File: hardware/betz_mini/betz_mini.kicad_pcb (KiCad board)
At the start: 2 copper layers, 17 parts, among them U1 stm32g474ceu6, U2 AS5047U, U3 IIS328DQ, U4 MP6540

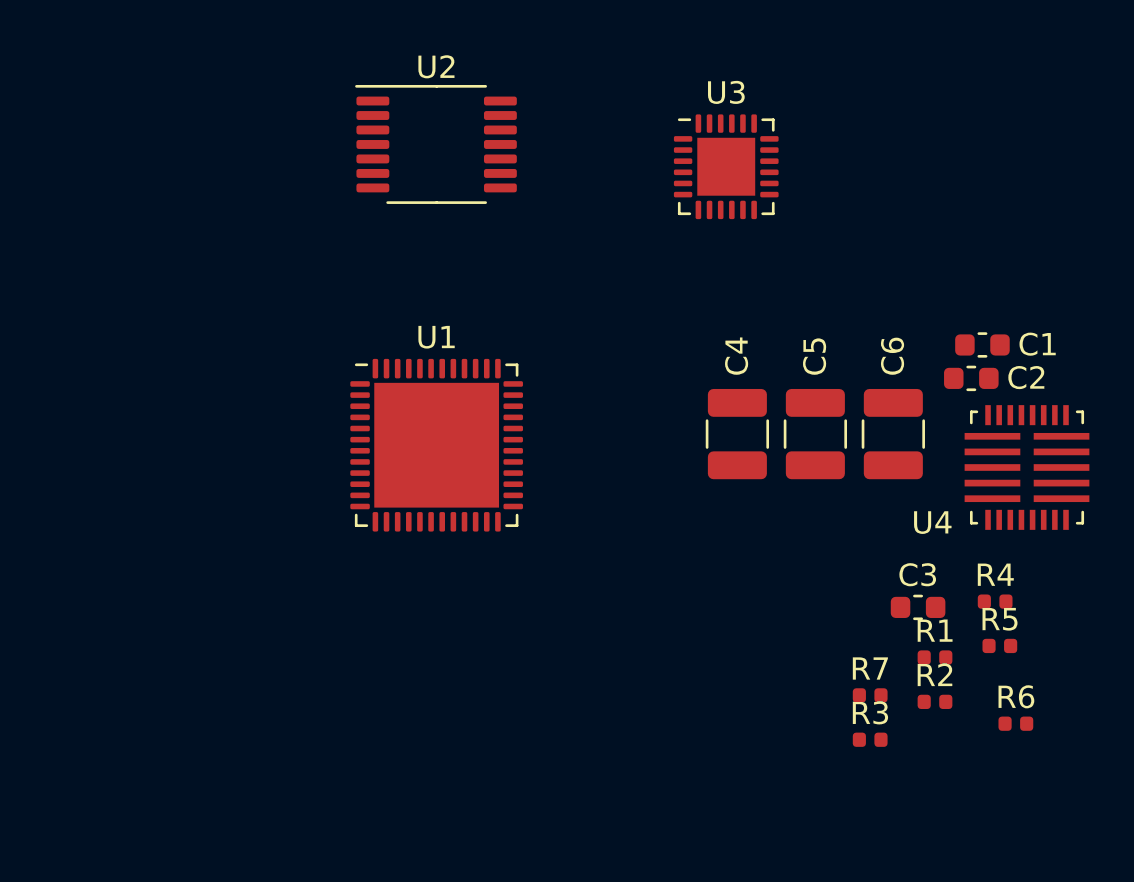
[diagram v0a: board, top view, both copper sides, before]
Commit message: WIP
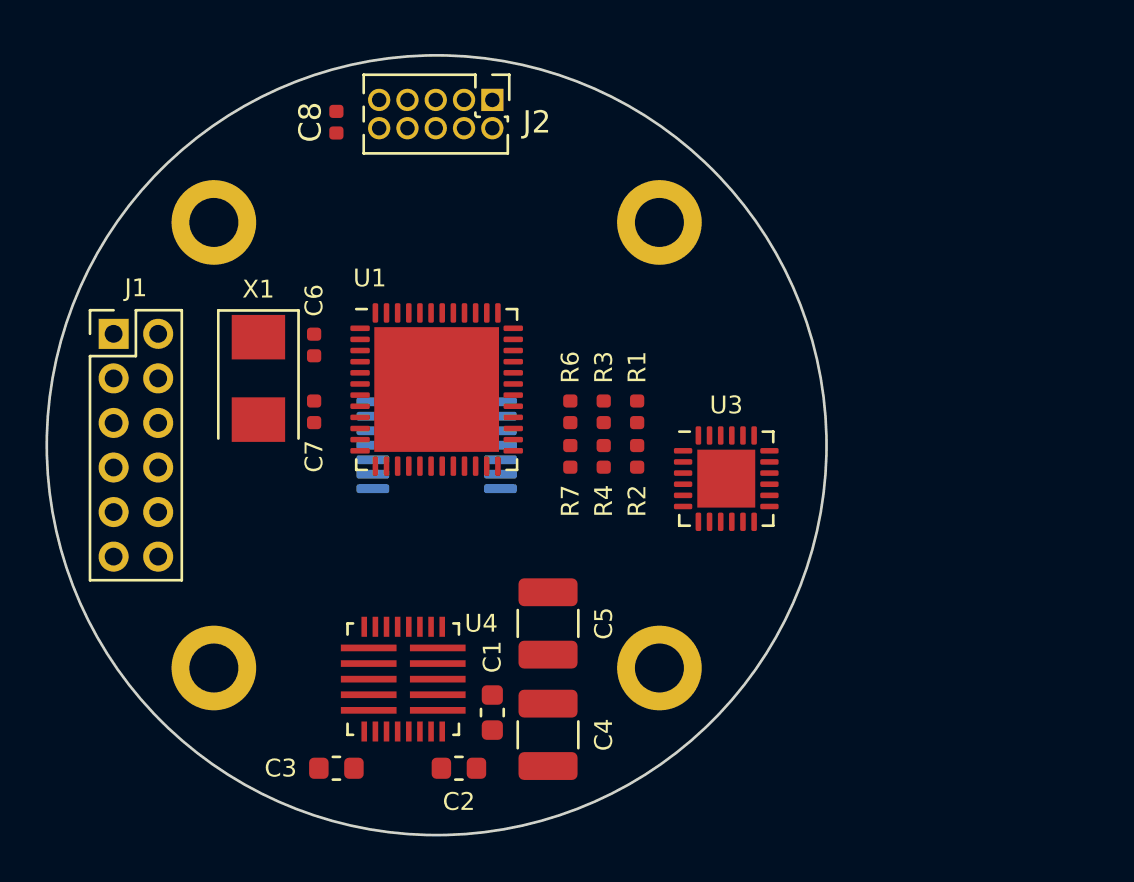
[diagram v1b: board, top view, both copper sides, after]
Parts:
- removed R5: 4k7, Resistor_SMD:R_0402_1005Metric
- added C7: 15p, Capacitor_SMD:C_0402_1005Metric, F.Cu at (144.5, 98.5)
- added C8: 100n, Capacitor_SMD:C_0402_1005Metric, F.Cu at (145.5, 85.5)
- added H1: MountingHole_Pad, MountingHole:MountingHole_2.2mm_M2_DIN965_Pad, F.Cu at (140.0, 90.0)
- added H2: MountingHole_Pad, MountingHole:MountingHole_2.2mm_M2_DIN965_Pad, F.Cu at (160.0, 90.0)
- added H3: MountingHole_Pad, MountingHole:MountingHole_2.2mm_M2_DIN965_Pad, F.Cu at (140.0, 110.0)
- added H4: MountingHole_Pad, MountingHole:MountingHole_2.2mm_M2_DIN965_Pad, F.Cu at (160.0, 110.0)
- added J1: upstairs, Connector_PinHeader_2.00mm:PinHeader_2x06_P2.00mm_Vertical, F.Cu at (135.5, 95.0)
- added J2: Conn_ARM_JTAG_SWD_10, Connector_PinHeader_1.27mm:PinHeader_2x05_P1.27mm_Vertical, F.Cu at (152.5, 84.5)
- added X1: 8 MHz, Crystal:Crystal_SMD_5032-2Pin_5.0x3.2mm, F.Cu at (142.0, 97.0)
- C4, C5: value 10u -> 22u
- C6: value 10u -> 15p; footprint Capacitor_SMD:C_1210_3225Metric -> Capacitor_SMD:C_0402_1005Metric
- U2: moved to B.Cu
- moved U4 29.6 mm to (148.5, 110.5), turned to -90 degrees
- moved C2 28.9 mm to (151.0, 114.5), turned to 0 degrees
- moved C1 27.5 mm to (152.5, 112.0), turned to -90 degrees
- moved C3 27.1 mm to (145.5, 114.5), turned to 180 degrees
- moved C6 26.3 mm to (144.5, 95.5), turned to -90 degrees
- moved R6 24.4 mm to (156.0, 98.5), turned to -90 degrees
- moved R3 19.0 mm to (157.5, 98.5), turned to -90 degrees
- moved R4 18.7 mm to (157.5, 100.5), turned to -90 degrees
- moved R1 17.3 mm to (159.0, 98.5), turned to -90 degrees
- moved R2 17.3 mm to (159.0, 100.5), turned to -90 degrees
- moved R7 17.2 mm to (156.0, 100.5), turned to -90 degrees
- moved C4 16.0 mm to (155.0, 113.0), turned to -90 degrees
- moved C5 14.7 mm to (155.0, 108.0)
- moved U3 14.0 mm to (163.0, 101.5)
- moved U2 13.5 mm to (150.0, 100.0)
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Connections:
- net Net-(C1-Pad2) renamed /VCP
- net Net-(C2-Pad1) renamed /CP1
- net Net-(C2-Pad2) renamed /CP2
- net Net-(C3-Pad1) renamed /VG
- C6 pad 1: VBUS -> Net-(C6-Pad1)
- U1 pad 1: Net-(U1-Pad1) -> +3V3
- U1 pad 23: Net-(U1-Pad23) -> +3V3
- U1 pad 35: Net-(U1-Pad35) -> +3V3
- U1 pad 36: Net-(U1-Pad36) -> /SWDIO
- U1 pad 37: Net-(U1-Pad37) -> /SWCLK
- U1 pad 48: Net-(U1-Pad48) -> +3V3
- U1 pad 5: Net-(U1-Pad5) -> Net-(C6-Pad1)
- U1 pad 7: Net-(U1-Pad7) -> /NRST
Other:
- board outline added: 35 x 35 mm
- copper layers 2 -> 4

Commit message: WIP. 35mm square
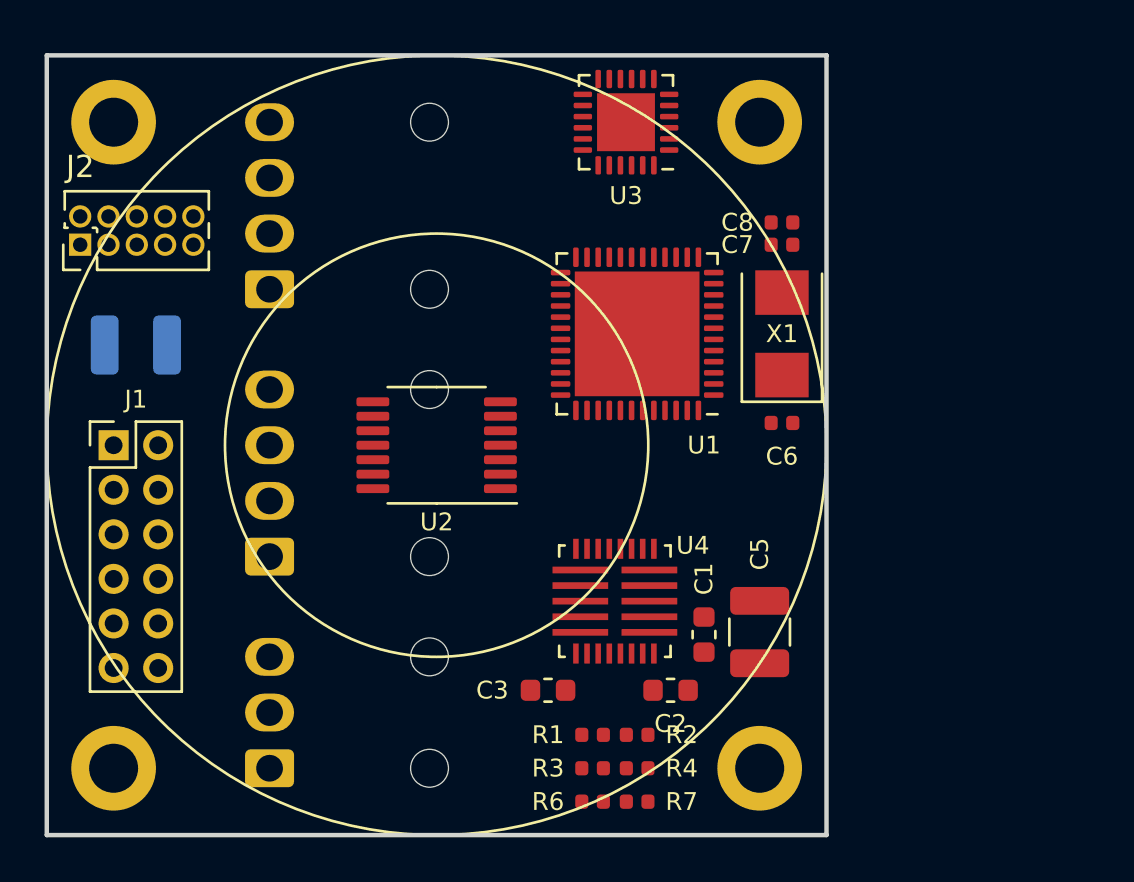
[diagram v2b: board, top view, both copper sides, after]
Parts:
- added REF**: Molex_Nano-Fit_105313-xx04_1x04_P2.50mm_Horizontal, Connector_Molex:Molex_Nano-Fit_105313-xx04_1x04_P2.50mm_Horizontal, B.Cu at (142.5, 93.0)
- added REF**: Molex_Nano-Fit_105313-xx04_1x04_P2.50mm_Horizontal, Connector_Molex:Molex_Nano-Fit_105313-xx04_1x04_P2.50mm_Horizontal, B.Cu at (142.5, 105.0)
- added REF**: Molex_Nano-Fit_105313-xx03_1x03_P2.50mm_Horizontal, Connector_Molex:Molex_Nano-Fit_105313-xx03_1x03_P2.50mm_Horizontal, B.Cu at (142.5, 114.5)
- C4: moved to B.Cu
- U2: moved to F.Cu
- moved C4 25.5 mm to (136.5, 95.5), turned to 180 degrees
- moved X1 23.6 mm to (165.5, 95.0), turned to 90 degrees
- moved C7 22.3 mm to (165.5, 91.0), turned to 0 degrees
- moved C6 21.3 mm to (165.5, 99.0), turned to 0 degrees
- moved C8 20.5 mm to (165.5, 90.0), turned to 0 degrees
- moved J2 19.6 mm to (134.0, 91.0), turned to 90 degrees
- moved R6 17.5 mm to (157.0, 116.0), turned to 0 degrees
- moved U3 16.6 mm to (158.5, 85.5), turned to 180 degrees
- moved R3 16.0 mm to (157.0, 114.5), turned to 0 degrees
- moved R7 15.8 mm to (159.0, 116.0), turned to 0 degrees
- moved R1 14.6 mm to (157.0, 113.0), turned to 0 degrees
- moved R4 14.1 mm to (159.0, 114.5), turned to 0 degrees
- moved R2 12.5 mm to (159.0, 113.0), turned to 0 degrees
- moved C1 10.1 mm to (162.0, 108.5)
- moved C2 10.1 mm to (160.5, 111.0)
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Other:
- outline, holes or cut-outs redrawn

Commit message: WIP detailing schematic and placement
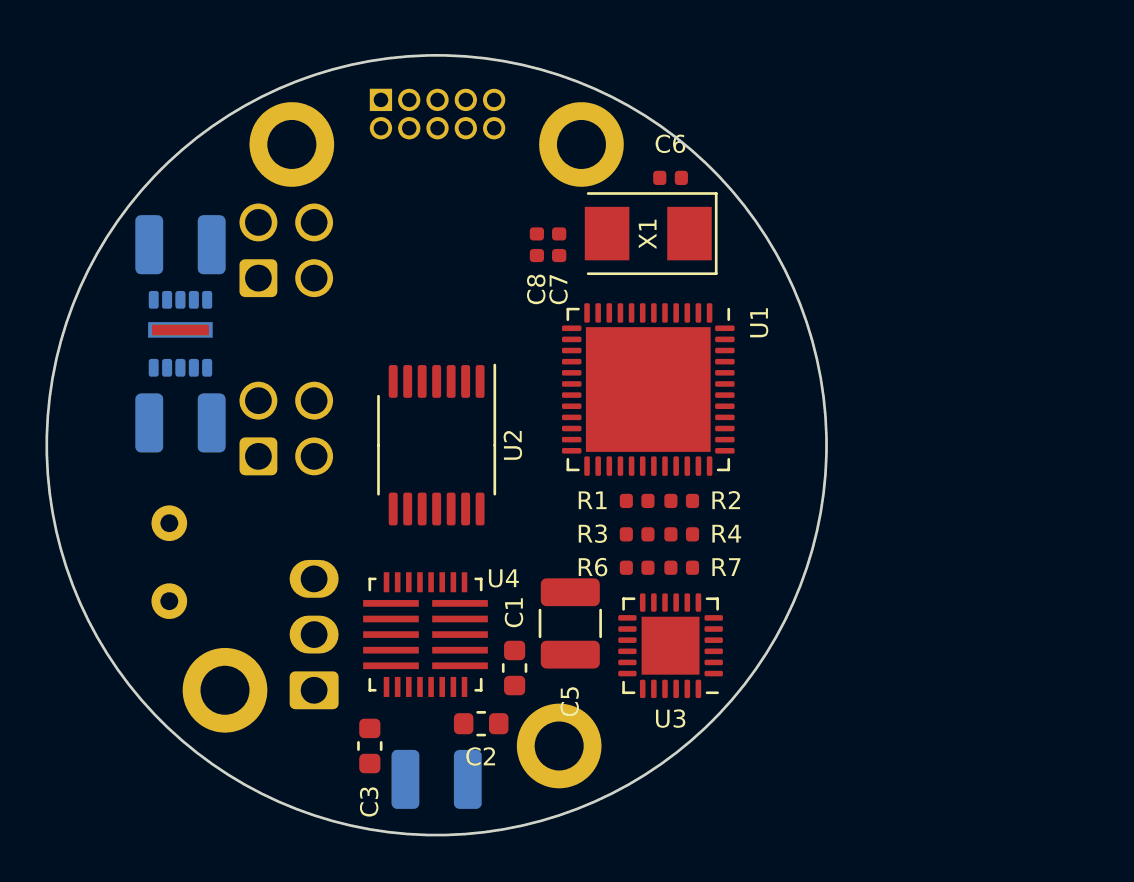
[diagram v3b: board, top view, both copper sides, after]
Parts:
- removed REF** (x2): Molex_Nano-Fit_105313-xx04_1x04_P2.50mm_Horizontal, Connector_Molex:Molex_Nano-Fit_105313-xx04_1x04_P2.50mm_Horizontal
- removed REF**: Molex_Nano-Fit_105313-xx03_1x03_P2.50mm_Horizontal, Connector_Molex:Molex_Nano-Fit_105313-xx03_1x03_P2.50mm_Horizontal
- added C10: 10u, Capacitor_SMD:C_1210_3225Metric, B.Cu at (150.0, 115.0)
- added C11: 47u, Capacitor_SMD:C_1210_3225Metric, B.Cu at (138.5, 99.0)
- added C9: 470u, Capacitor_THT:C_Radial_D8.0mm_H11.5mm_P3.50mm, B.Cu at (138.0, 103.5)
- added J2: downstream, Connector_Molex:Molex_Nano-Fit_105314-xx04_2x02_P2.50mm_Horizontal, B.Cu at (142.0, 100.5)
- added J4: BLDC, Connector_Molex:Molex_Nano-Fit_105313-xx03_1x03_P2.50mm_Horizontal, B.Cu at (144.5, 111.0)
- added U5: LMZM23601V3, Package_LGA:Texas_SIL0010A_MicroSiP-10-1EP_3.8x3mm_P0.6mm_EP0.7x2.9mm_ThermalVias, B.Cu at (138.5, 95.0)
- J1: value upstairs -> upstream; footprint Connector_PinHeader_2.00mm:PinHeader_2x06_P2.00mm_Vertical -> Connector_Molex:Molex_Nano-Fit_105314-xx04_2x02_P2.50mm_Horizontal; moved to B.Cu
- J3: renamed from J2; value Conn_ARM_JTAG_SWD_10 -> ARM SWD; moved to B.Cu
- moved U3 23.6 mm to (160.5, 109.0)
- moved J3 15.0 mm to (147.5, 84.5), turned to -90 degrees
- moved C6 12.1 mm to (160.5, 88.0), turned to 180 degrees
- moved C8 11.0 mm to (154.5, 91.0), turned to 90 degrees
- moved R1 10.7 mm to (159.0, 102.5)
- moved R2 10.7 mm to (161.0, 102.5)
- moved R3 10.7 mm to (159.0, 104.0)
- moved R4 10.7 mm to (161.0, 104.0)
- moved R6 10.7 mm to (159.0, 105.5)
- moved R7 10.7 mm to (161.0, 105.5)
- moved C7 10.0 mm to (155.5, 91.0), turned to 90 degrees
- moved J1 9.92 mm to (142.0, 92.5)
- moved H4 9.06 mm to (155.5, 113.5)
- moved C1 8.63 mm to (153.5, 110.0)
- moved C2 8.63 mm to (152.0, 112.5)
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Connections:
- net /RX renamed Net-(J1-Pad3)
- J1 pad 1: +3V3 -> VBUS
- J1 pad 2: /TX -> GND
- J1 pad 4: GND -> Net-(J1-Pad4)
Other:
- outline, holes or cut-outs redrawn
